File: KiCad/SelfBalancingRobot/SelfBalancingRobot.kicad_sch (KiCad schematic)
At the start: 5 parts, among them U1 ESP32_NODEMCU, U2 GY-521

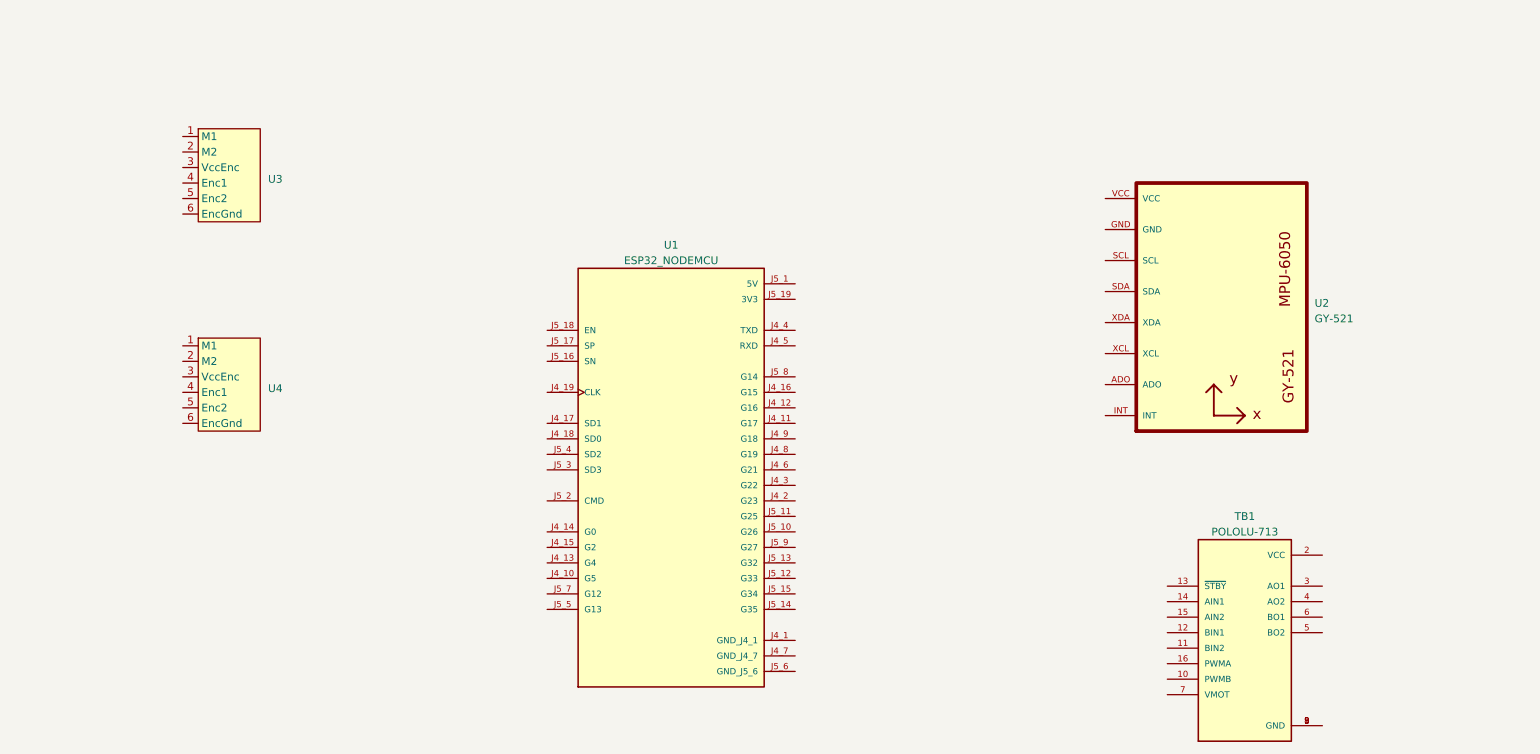
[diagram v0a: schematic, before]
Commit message: kicad
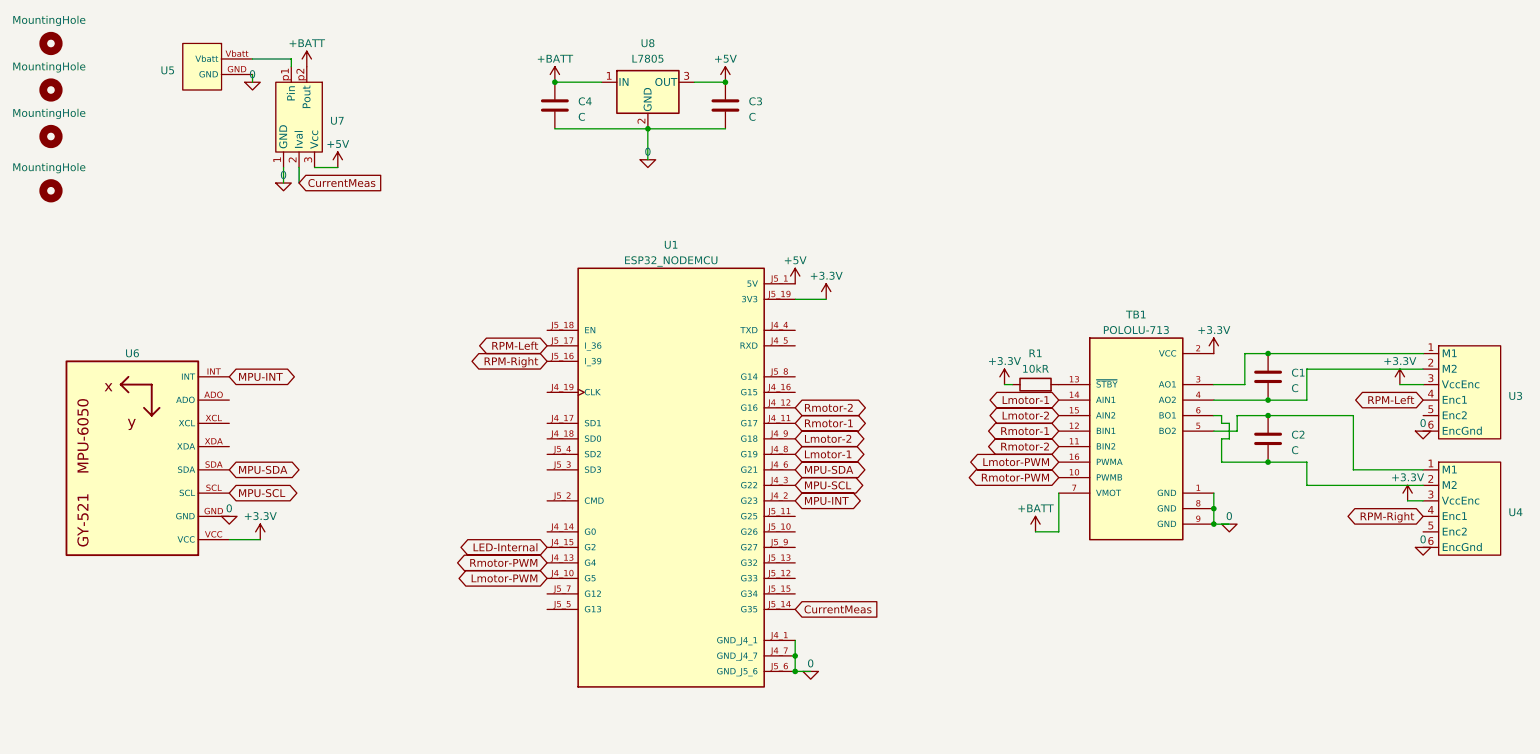
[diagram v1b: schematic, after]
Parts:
- removed U2: GY-521, GY-521, symbol GY-521:GY-521
- added C1, C2: C, Capacitor_THT:C_Disc_D6.0mm_W4.4mm_P5.00mm, symbol Device:C
- added C3, C4: C, Capacitor_THT:CP_Radial_D6.3mm_P2.50mm, symbol Device:C
- added H1, H2, H3, H4: MountingHole, MountingHole:MountingHole_3.2mm_M3_DIN965_Pad_TopBottom, symbol Mechanical:MountingHole
- added R1: 10kR, Resistor_THT:R_Axial_DIN0204_L3.6mm_D1.6mm_P7.62mm_Horizontal, symbol Device:R
- added U5: ~, 0_Footprints:BatteryConnector, symbol 0_Library:BatteryConnector
- added U6: ~, 0_Footprints:MPU-6050-External, symbol 0_Library:MPU-6050
- added U7: ~, 0_Footprints:CurrentMeter, symbol 0_Library:CurrentMeter
- added U8: L7805, Package_TO_SOT_THT:TO-220-3_Horizontal_TabDown, symbol Regulator_Linear:L7805
- U3, U4: footprint (none) -> 0_Footprints:V-TecMotorHeader
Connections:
- net at U4.1 (M1): now also TB1.5 (BO2), C2.1
- net at U4.2 (M2): now also TB1.6 (BO1), C2.2
- net +3.3V: now reaches U4.3 (VccEnc)
- net +3.3V: now also TB1.2 (VCC), U1.J5_19 (3V3), U3.3 (VccEnc), R1.1, U6.VCC
- net RPM-Right: now reaches U4.4 (Enc1)
- net RPM-Right: now also U1.J5_16 (I_39)
- net 0: now reaches U4.6 (EncGnd)
- net 0: now also TB1.1 (GND), TB1.8 (GND), TB1.9 (GND), U1.J4_1 (GND_J4_1), U1.J4_7 (GND_J4_7), U1.J5_6 (GND_J5_6), U3.6 (EncGnd), C3.2, C4.2, U5.GND, U6.GND, U7.1 (GND), U8.2 (GND)
- net Lmotor-PWM: now reaches U1.J4_10 (G5)
- net Lmotor-PWM: now also TB1.16 (PWMA)
- net Rmotor-1: now reaches U1.J4_11 (G17)
- net Rmotor-1: now also TB1.12 (BIN1)
- net Rmotor-2: now reaches U1.J4_12 (G16)
- net Rmotor-2: now also TB1.11 (BIN2)
- net Rmotor-PWM: now reaches U1.J4_13 (G4)
- net Rmotor-PWM: now also TB1.10 (PWMB)
- net LED-Internal: now reaches U1.J4_15 (G2)
- net MPU-INT: now reaches U1.J4_2 (G23)
- net MPU-INT: now also U6.INT
- net MPU-SCL: now reaches U1.J4_3 (G22)
- net MPU-SCL: now also U6.SCL
- net MPU-SDA: now reaches U1.J4_6 (G21)
- net MPU-SDA: now also U6.SDA
- net Lmotor-1: now reaches U1.J4_8 (G19)
- net Lmotor-1: now also TB1.14 (AIN1)
- net Lmotor-2: now reaches U1.J4_9 (G18)
- net Lmotor-2: now also TB1.15 (AIN2)
- net +5V: now reaches U1.J5_1 (5V)
- net +5V: now also C3.1, U7.3 (Vcc), U8.3 (OUT)
- net CurrentMeas: now reaches U1.J5_14 (G35)
- net CurrentMeas: now also U7.2 (Ival)
- net RPM-Left: now reaches U1.J5_17 (I_36)
- net RPM-Left: now also U3.4 (Enc1)
- net at TB1.13 (~{STBY}): now also R1.2
- net at TB1.3 (AO1): now also U3.1 (M1), C1.1
- net at TB1.4 (AO2): now also U3.2 (M2), C1.2
- net +BATT: now reaches TB1.7 (VMOT)
- net +BATT: now also C4.1, U7.p2 (Pout), U8.1 (IN)
- new net: U5.Vbatt, U7.p1 (Pin)
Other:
- moved on the sheet: U3, U4
